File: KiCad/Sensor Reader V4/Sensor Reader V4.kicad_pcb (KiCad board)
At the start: 2 copper layers, 43 x 62.5 mm, 47 parts, among them J1 USB_C_Receptacle_USB2.0_16P, J10 L_I/B1_Out, J11 B1_Net/B2_In, J12 B2_Net/B2_Out, J13 AIN_4, J14 AIN_5, J15 5V_Input, J16 3.3V_Output, J6 Exposed_UART, J7 Batt1_V, J8 Batt2_V, J9 M_OUT/B1_In, SW1 BOOT_Btn, SW2 EN_Btn, U1 AMS1117-3.3, U2 USBLC6-2P6, U3 ADS8688, U4 ESP32-C3-WROOM-02

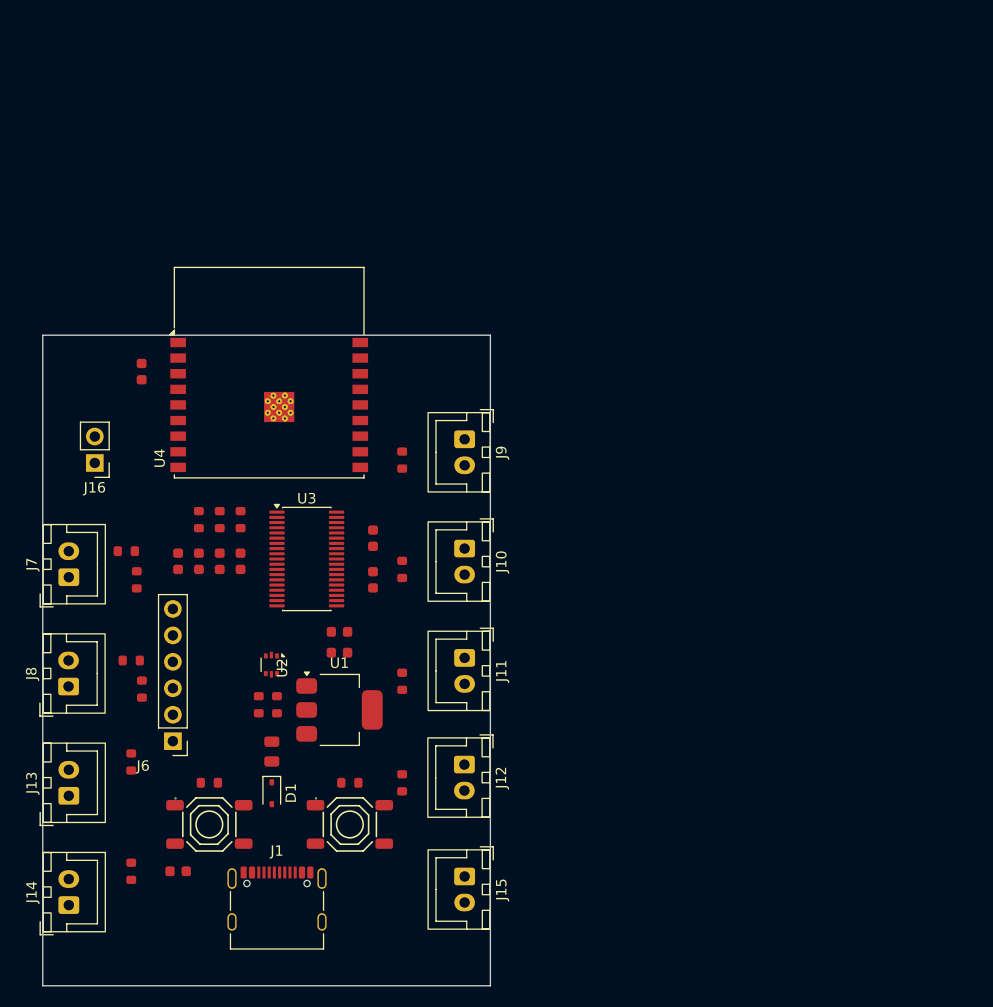
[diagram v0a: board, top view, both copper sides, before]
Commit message: pdb
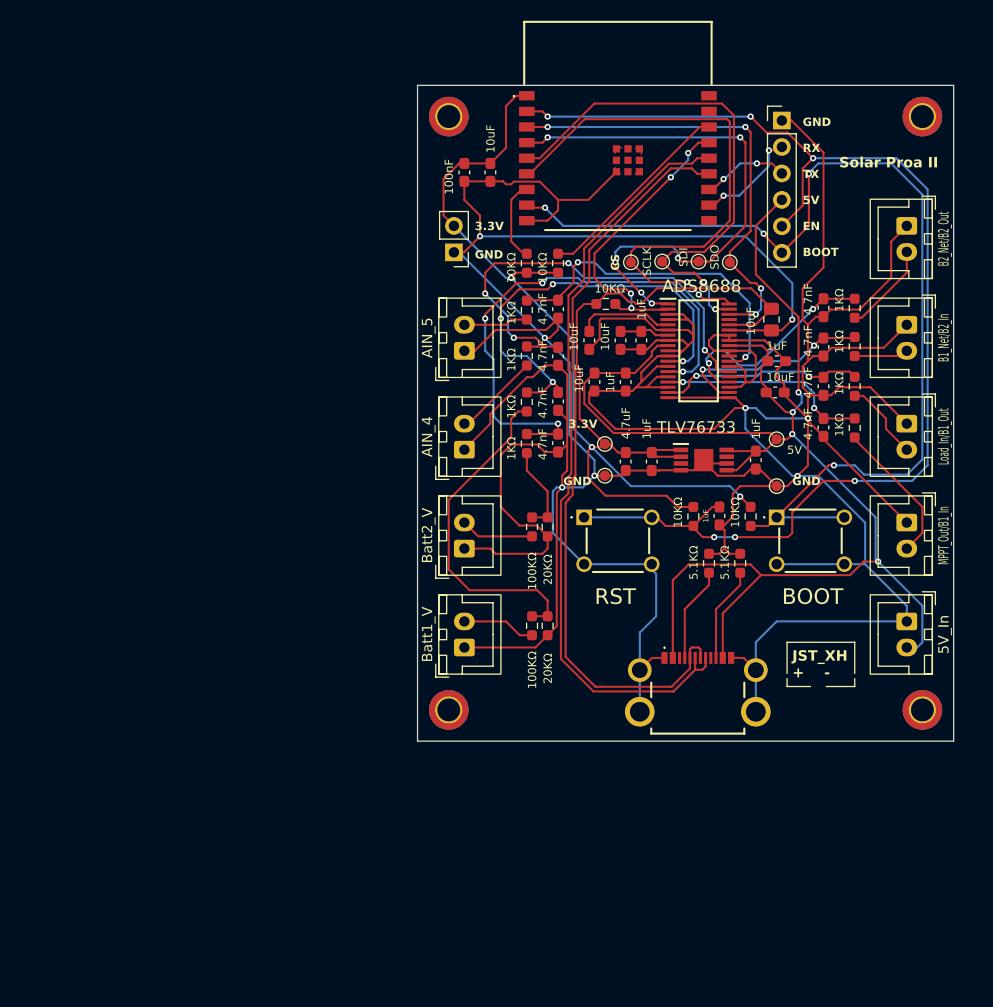
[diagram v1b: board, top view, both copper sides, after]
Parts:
- removed C1: 47uF, PCM_JLCPCB:C_0805
- removed D1: 1N5819WS, Diode_SMD:D_SOD-323
- removed J1: USB_C_Receptacle_USB2.0_16P, Connector_USB:USB_C_Receptacle_Palconn_UTC16-G
- removed J10: L_I/B1_Out, Connector_JST:JST_XH_B2B-XH-A_1x02_P2.50mm_Vertical
- removed J11: B1_Net/B2_In, Connector_JST:JST_XH_B2B-XH-A_1x02_P2.50mm_Vertical
- removed J12: B2_Net/B2_Out, Connector_JST:JST_XH_B2B-XH-A_1x02_P2.50mm_Vertical
- removed J13: AIN_4, Connector_JST:JST_XH_B2B-XH-A_1x02_P2.50mm_Vertical
- removed J14: AIN_5, Connector_JST:JST_XH_B2B-XH-A_1x02_P2.50mm_Vertical
- removed J15: 5V_Input, Connector_JST:JST_XH_B2B-XH-A_1x02_P2.50mm_Vertical
- removed J7: Batt1_V, Connector_JST:JST_XH_B2B-XH-A_1x02_P2.50mm_Vertical
- removed J8: Batt2_V, Connector_JST:JST_XH_B2B-XH-A_1x02_P2.50mm_Vertical
- removed J9: M_OUT/B1_In, Connector_JST:JST_XH_B2B-XH-A_1x02_P2.50mm_Vertical
- removed U1: AMS1117-3.3, Package_TO_SOT_SMD:SOT-223-3_TabPin2
- removed U2: USBLC6-2P6, Package_TO_SOT_SMD:SOT-666
- removed U4: ESP32-C3-WROOM-02, RF_Module:ESP32-C3-WROOM-02
- added 5V_In: 5V_Input, Connector_JST:JST_XH_B2B-XH-A_1x02_P2.50mm_Vertical, F.Cu at (164.5, 89.5)
- added AIN_4: AIN_4, Connector_JST:JST_XH_B2B-XH-A_1x02_P2.50mm_Vertical, F.Cu at (122.0, 73.0)
- added AIN_5: AIN_5, Connector_JST:JST_XH_B2B-XH-A_1x02_P2.50mm_Vertical, F.Cu at (122.0, 63.5)
- added B1_Net/B2_In: B1_Net/B2_In, Connector_JST:JST_XH_B2B-XH-A_1x02_P2.50mm_Vertical, F.Cu at (164.5, 61.0)
- added B2_Net/B2_Out: B2_Net/B2_Out, Connector_JST:JST_XH_B2B-XH-A_1x02_P2.50mm_Vertical, F.Cu at (164.5, 51.5)
- added Batt1_V: Batt1_V, Connector_JST:JST_XH_B2B-XH-A_1x02_P2.50mm_Vertical, F.Cu at (122.0, 92.0)
- added Batt2_V: Batt2_V, Connector_JST:JST_XH_B2B-XH-A_1x02_P2.50mm_Vertical, F.Cu at (122.0, 82.5)
- added C13: 1uF, Capacitor_SMD:C_0603_1608Metric_Pad1.08x0.95mm_HandSolder, F.Cu at (140.0, 74.1)
- added C14: 4.7nF, Capacitor_SMD:C_0603_1608Metric_Pad1.08x0.95mm_HandSolder, F.Cu at (131.0, 59.5)
- added C15: 4.7nF, Capacitor_SMD:C_0603_1608Metric_Pad1.08x0.95mm_HandSolder, F.Cu at (131.0, 68.4)
- added C16: 4.7nF, Capacitor_SMD:C_0603_1608Metric_Pad1.08x0.95mm_HandSolder, F.Cu at (131.0, 72.4)
- added C17: 4.7nF, Capacitor_SMD:C_0603_1608Metric_Pad1.08x0.95mm_HandSolder, F.Cu at (156.5, 63.1)
- added C18: 4.7nF, Capacitor_SMD:C_0603_1608Metric_Pad1.08x0.95mm_HandSolder, F.Cu at (156.5, 59.4)
- added C19: 4.7nF, Capacitor_SMD:C_0603_1608Metric_Pad1.08x0.95mm_HandSolder, F.Cu at (131.0, 64.0)
- added C2: 1uF, Capacitor_SMD:C_0603_1608Metric_Pad1.08x0.95mm_HandSolder, F.Cu at (150.0, 74.0)
- added C20: 10uF, Capacitor_SMD:C_0603_1608Metric_Pad1.08x0.95mm_HandSolder, F.Cu at (134.5, 66.5)
- added C21: 4.7nF, Capacitor_SMD:C_0603_1608Metric_Pad1.08x0.95mm_HandSolder, F.Cu at (156.5, 70.9)
- added C22: 4.7nF, Capacitor_SMD:C_0603_1608Metric_Pad1.08x0.95mm_HandSolder, F.Cu at (156.5, 66.9)
- added C23: 10uF, Capacitor_SMD:C_0603_1608Metric_Pad1.08x0.95mm_HandSolder, F.Cu at (122.0, 46.4)
- added CS: TestPoint, TestPoint:TestPoint_Pad_D1.0mm, F.Cu at (138.0, 55.0)
- added IC1: TLV76733DGNR, SamacSys_Parts:SOP65P490X110-9N, F.Cu at (145.0, 74.0)
- added IC2: ESP32-C3-WROOM-02-H4, SamacSys_Parts:ESP32C3WROOM02H4, F.Cu at (127.2, 51.9)
- added J2: UJ20-C-H-G-MSMT-2B-P16-TR, SamacSys_Parts:UJ20CHGMSMT2BP16TR, F.Cu at (144.4, 98.2)
- added Load_In/B1_Out: L_I/B1_Out, Connector_JST:JST_XH_B2B-XH-A_1x02_P2.50mm_Vertical, F.Cu at (164.5, 70.5)
- added MPPT_Out/B1_In: M_OUT/B1_In, Connector_JST:JST_XH_B2B-XH-A_1x02_P2.50mm_Vertical, F.Cu at (164.5, 80.0)
- added R14: 1kΩ, Resistor_SMD:R_0603_1608Metric_Pad0.98x0.95mm_HandSolder, F.Cu at (128.0, 68.4)
- added R15: 1kΩ, Resistor_SMD:R_0603_1608Metric_Pad0.98x0.95mm_HandSolder, F.Cu at (128.0, 72.4)
- added REF**: MountingHole_2.2mm_M2_DIN965_Pad_TopBottom, MountingHole:MountingHole_2.2mm_M2_DIN965_Pad_TopBottom, F.Cu at (166.0, 41.0)
- added REF**: MountingHole_2.2mm_M2_DIN965_Pad_TopBottom, MountingHole:MountingHole_2.2mm_M2_DIN965_Pad_TopBottom, F.Cu at (166.0, 98.0)
- added REF**: MountingHole_2.2mm_M2_DIN965_Pad_TopBottom, MountingHole:MountingHole_2.2mm_M2_DIN965_Pad_TopBottom, F.Cu at (120.5, 41.0)
- added REF**: MountingHole_2.2mm_M2_DIN965_Pad_TopBottom, MountingHole:MountingHole_2.2mm_M2_DIN965_Pad_TopBottom, F.Cu at (120.5, 98.0)
- added SCLK: TestPoint, TestPoint:TestPoint_Pad_D1.0mm, F.Cu at (141.0, 54.9)
- added SDI: TestPoint, TestPoint:TestPoint_Pad_D1.0mm, F.Cu at (144.5, 54.9)
- added SDO: TestPoint, TestPoint:TestPoint_Pad_D1.0mm, F.Cu at (147.5, 55.0)
- added TP1: TestPoint, TestPoint:TestPoint_Pad_D1.0mm, F.Cu at (135.5, 72.5)
- added TP2: TestPoint, TestPoint:TestPoint_Pad_D1.0mm, F.Cu at (135.5, 75.5)
- added TP3: TestPoint, TestPoint:TestPoint_Pad_D1.0mm, F.Cu at (152.0, 72.0)
- added TP8: TestPoint, TestPoint:TestPoint_Pad_D1.0mm, F.Cu at (152.0, 76.5)
- C10, C9: value 10nF -> 1uF; footprint PCM_JLCPCB:C_0603 -> Capacitor_SMD:C_0603_1608Metric_Pad1.08x0.95mm_HandSolder
- C11: value 10nF -> 10uF; footprint PCM_JLCPCB:C_0603 -> Capacitor_SMD:C_0805_2012Metric_Pad1.18x1.45mm_HandSolder
- C12: value 100nF -> 10uF; footprint PCM_JLCPCB:C_0603 -> Capacitor_SMD:C_0603_1608Metric_Pad1.08x0.95mm_HandSolder
- C3, C6, C7: footprint PCM_JLCPCB:C_0603 -> Capacitor_SMD:C_0603_1608Metric_Pad1.08x0.95mm_HandSolder
- C4: value 100nF -> 1uF; footprint PCM_JLCPCB:C_0603 -> Capacitor_SMD:C_0603_1608Metric_Pad1.08x0.95mm_HandSolder
- C5: value 10nF -> 10uF; footprint PCM_JLCPCB:C_0603 -> Capacitor_SMD:C_0603_1608Metric_Pad1.08x0.95mm_HandSolder
- C8: value 1uF -> 10uF; footprint PCM_JLCPCB:C_0603 -> Capacitor_SMD:C_0603_1608Metric_Pad1.08x0.95mm_HandSolder
- R1, R10, R11, R12, R13, R16, R17, R18, R19, R2, R3, R4, R5, R6, R7, R8, R9: footprint PCM_JLCPCB:R_0603 -> Resistor_SMD:R_0603_1608Metric_Pad0.98x0.95mm_HandSolder
- SW1, SW2: footprint PCM_JLCPCB:SW-SMD_4P-L5.1-W5.1-P3.70-LS6.5-TL-2 -> SamacSys_Parts:TS0266100BK100LCRD
- U3: footprint Package_SO:TSSOP-38_4.4x9.7mm_P0.5mm -> SamacSys_Parts:SOP50P640X120-38N
- moved J6 83.5 mm to (152.5, 41.4), turned to 0 degrees
- moved R13 66.0 mm to (128.0, 59.6)
- moved R11 63.0 mm to (159.5, 59.4)
- moved C4 62.2 mm to (146.5, 79.4), turned to -90 degrees
- moved R12 54.5 mm to (128.0, 64.0)
- moved R10 54.1 mm to (159.5, 63.1)
- moved R3 53.1 mm to (144.0, 79.4), turned to -90 degrees
- moved SW1 50.5 mm to (152.0, 79.5)
- moved C12 48.8 mm to (151.9, 67.5)
- moved R1 48.2 mm to (148.5, 83.9)
- moved C7 47.5 mm to (139.0, 62.5)
- moved R9 46.9 mm to (159.5, 66.9)
- moved SW2 46.5 mm to (133.5, 79.5)
- moved R4 46.2 mm to (149.5, 79.4), turned to -90 degrees
- moved C5 44.8 mm to (134.0, 62.5)
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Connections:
- C12 pad 1: GND -> +5V
- C12 pad 2: +3.3V -> GND
- R16 pad 2: Net-(U3-AIN_6P) -> Net-(R14-Pad1)
- R17 pad 1: Net-(U3-AIN_6P) -> Net-(R14-Pad1)
- R18 pad 2: Net-(U3-AIN_7P) -> Net-(R15-Pad1)
- R19 pad 1: Net-(U3-AIN_7P) -> Net-(R15-Pad1)
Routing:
- net GND: track 0.00 -> 529.0 mm, vias 0 -> 8
- net +5V: track 0.00 -> 144.8 mm, vias 0 -> 4
- net +3.3V: track 0.00 -> 133.9 mm, vias 0 -> 3
- net EN: track 0.00 -> 117.1 mm, vias 0 -> 6
- net BOOT: track 0.00 -> 99.5 mm, vias 0 -> 4
- net USB_D+: track 0.00 -> 74.3 mm
- net USB_D-: track 0.00 -> 72.9 mm
- net CS: track 0.00 -> 54.5 mm, vias 0 -> 2
- net SDI: track 0.00 -> 52.7 mm, vias 0 -> 6
- net Net-(U3-AIN_7P): track 0.00 -> 52.4 mm, vias 0 -> 4
- net SCLK: track 0.00 -> 50.7 mm, vias 0 -> 2
- net Net-(U3-AIN_4P): track 0.00 -> 44.7 mm, vias 0 -> 4
- net SDO: track 0.00 -> 44.3 mm, vias 0 -> 4
- net Net-(U3-AIN_6P): track 0.00 -> 42.1 mm, vias 0 -> 4
- net Net-(U3-AIN_5P): track 0.00 -> 32.9 mm, vias 0 -> 2
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- added copper zone on F.Cu, net GND
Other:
- board size 43 x 62.5 mm -> 51.5 x 63 mm
- board text added: "100KΩ"
- board text added: "100nF"
- board text added: "10KΩ"
- board text added: "10uF"
- board text added: "1KΩ"
- board text added: "1uF"
- board text added: "20KΩ"
- board text added: "3.3V"
- board text added: "4.7nF"
- board text added: "4.7uF"
- board text added: "5.1KΩ"
- board text added: "5V"
- board text added: "ADS8688"
- board text added: "BOOT"
- board text added: "EN"
- board text added: "GND"
- board text added: "JST_XH + -"
- board text added: "RST"
- board text added: "RX"
- board text added: "Solar Proa II"
- board text added: "TLV76733"
- board text added: "TX"
